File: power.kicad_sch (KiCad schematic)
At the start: 26 parts, among them U3 EA3036, U8 TLV71312PDBV

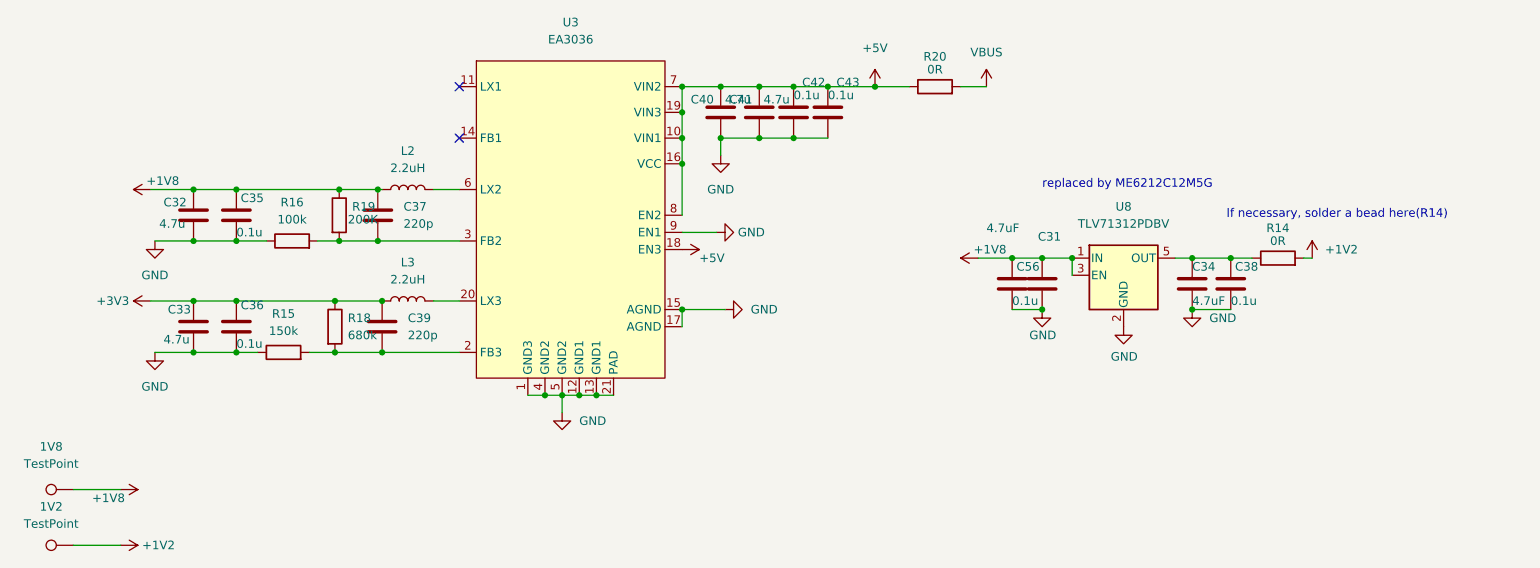
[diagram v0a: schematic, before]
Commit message: update 2.0
Signed-off-by: huangzzk <huangcmzzk@gmail.com>
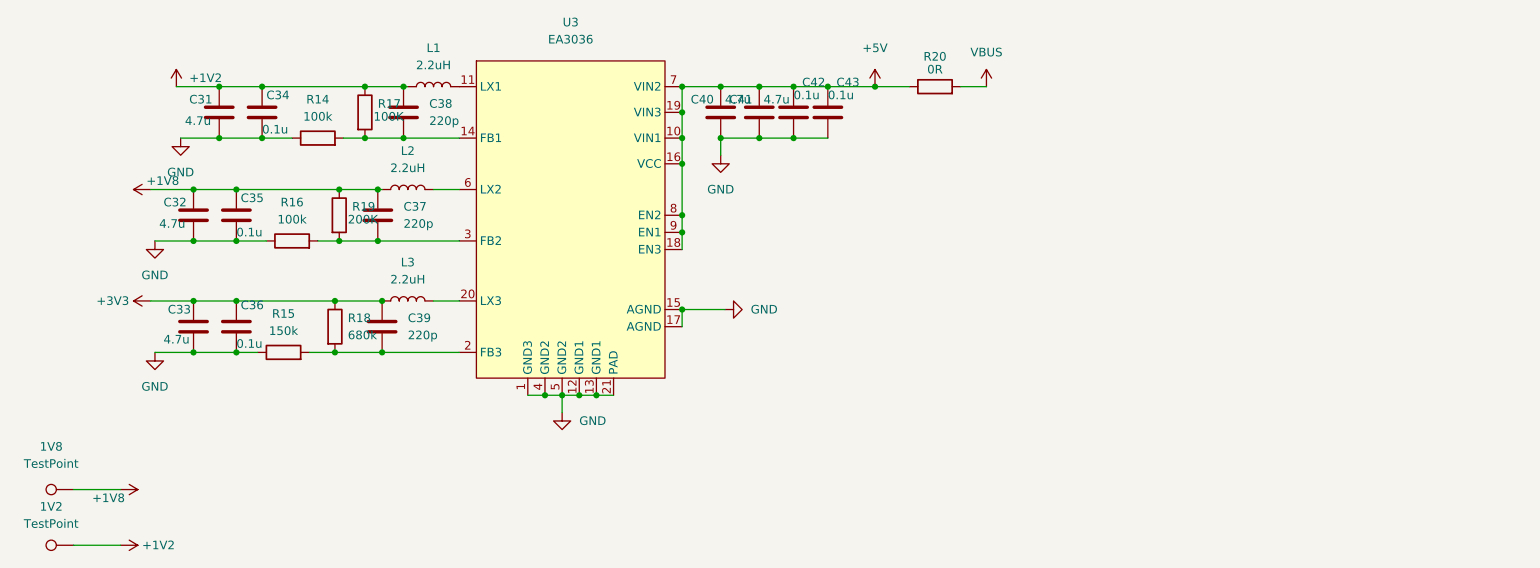
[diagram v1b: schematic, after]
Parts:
- removed C56: 0.1u, Capacitor_SMD:C_0402_1005Metric, symbol Device:C
- removed U8: TLV71312PDBV, Package_TO_SOT_SMD:SOT-23-5, symbol Regulator_Linear:TLV71312PDBV
- added L1: 2.2uH, Inductor_SMD:L_Abracon_ASPI-3012S, symbol Device:L
- added R17: 100K, Resistor_SMD:R_0402_1005Metric, symbol Device:R
- C31: value 4.7uF -> 4.7u
- C34: value 4.7uF -> 0.1u
- C38: value 0.1u -> 220p
- R14: value 0R -> 100k
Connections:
- net +1V2: now also C31.1, C34.1, C38.1, L1.1, R17.1; no longer R14.2
- net +1V8: no longer C31.1
- net +5V: now also U3.9 (EN1)
- net GND: now also R14.1; no longer C38.2, U3.9 (EN1)
- net at U3.11 (LX1): now also L1.2
- net at U3.14 (FB1): now also C38.2, R14.2, R17.2
- no-connect marks 2 -> 0
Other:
- note removed: "If necessary, solder a bead here(R14)"
- note removed: "replaced by ME6212C12M5G"
